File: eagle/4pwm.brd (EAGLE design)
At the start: 16.5 x 15.2 mm, 17 parts, among them U1 Tiny85-20-SMT

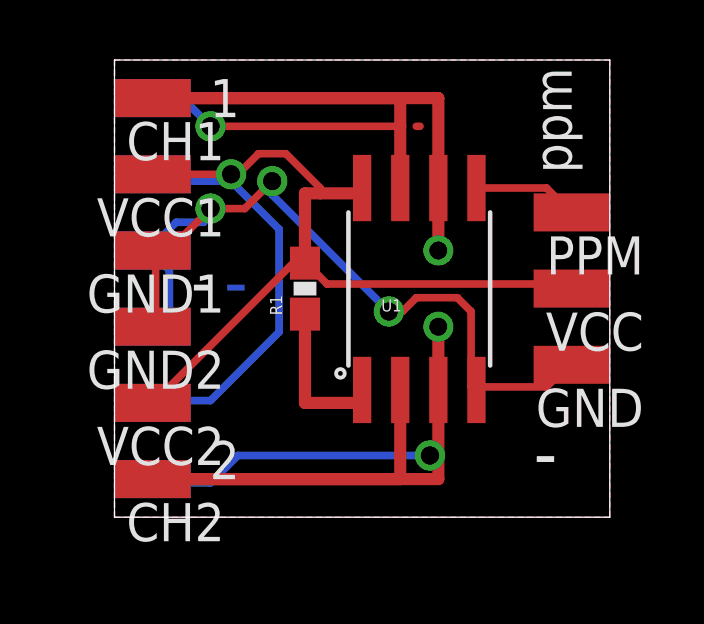
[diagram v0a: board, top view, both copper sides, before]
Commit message: Did some manual routing on the breakout
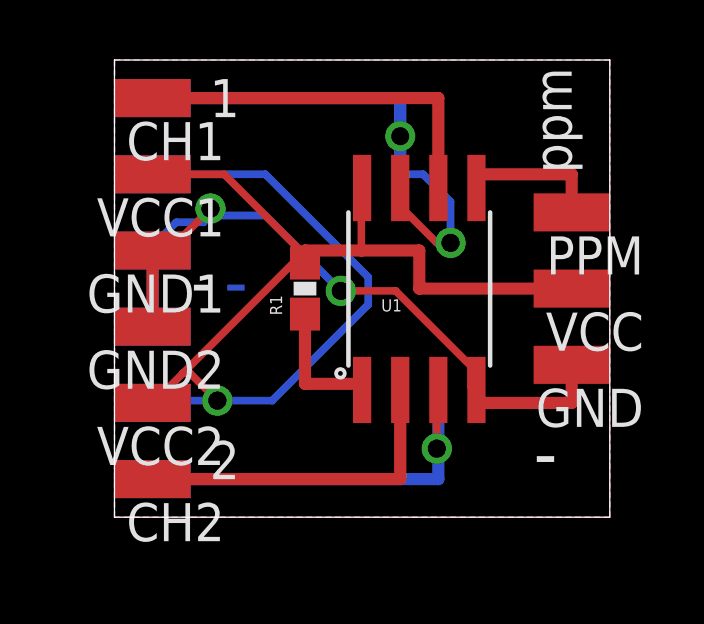
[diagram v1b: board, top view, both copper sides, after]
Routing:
- net N$7: track 24.6 -> 14.5 mm
- net VCC: track 41.2 -> 45.9 mm
- net N$5: track 19.9 -> 17.5 mm
- net N$4: track 14.6 -> 12.5 mm
- net GND: track 28.8 -> 27.0 mm, vias 3 -> 2
- net N$3: track 3.51 -> 4.90 mm
- net N$1: track 5.30 -> 4.43 mm
